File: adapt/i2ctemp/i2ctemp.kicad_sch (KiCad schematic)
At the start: 5 parts, among them J1 Conn_01x04_Pin, U1 TMP102xxDRL

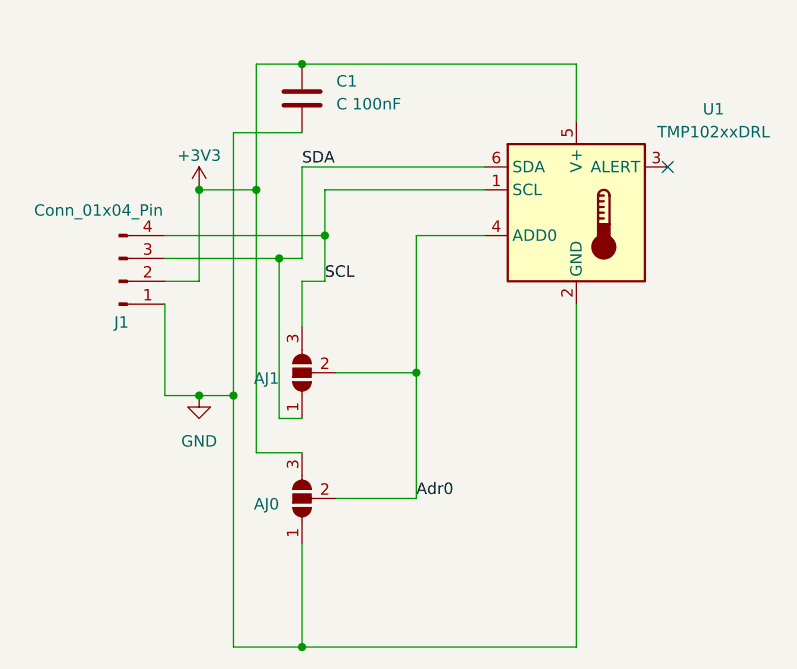
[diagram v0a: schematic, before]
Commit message: A host of un-logged changes
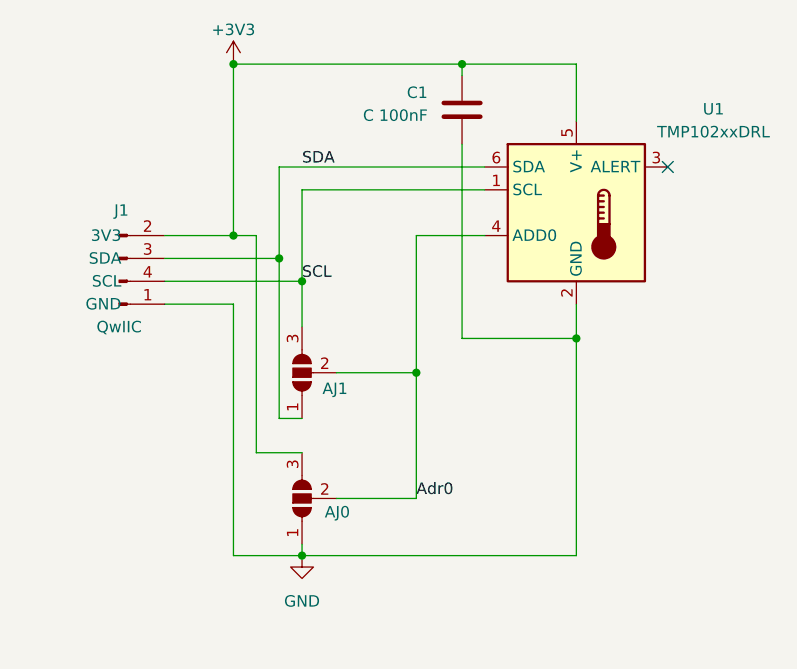
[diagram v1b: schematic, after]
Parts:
- J1: value Conn_01x04_Pin -> QwIIC; symbol Connector:Conn_01x04_Pin -> localstuff:QwIIC_h
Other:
- moved on the sheet: C1
